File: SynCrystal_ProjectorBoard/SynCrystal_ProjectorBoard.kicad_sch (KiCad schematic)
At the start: 20 parts, among them J10 Screw_Terminal_01x03, J11 to DIN Traces, J5 Relais Board, J6 uC Cable, J7 to DIN Connector, J8 to Motor Ctrl PCB, J9 to Motor Controller Hat, SW6 SW_SPDT, U10 AP63205WU, U9 TS5A3357DCUR

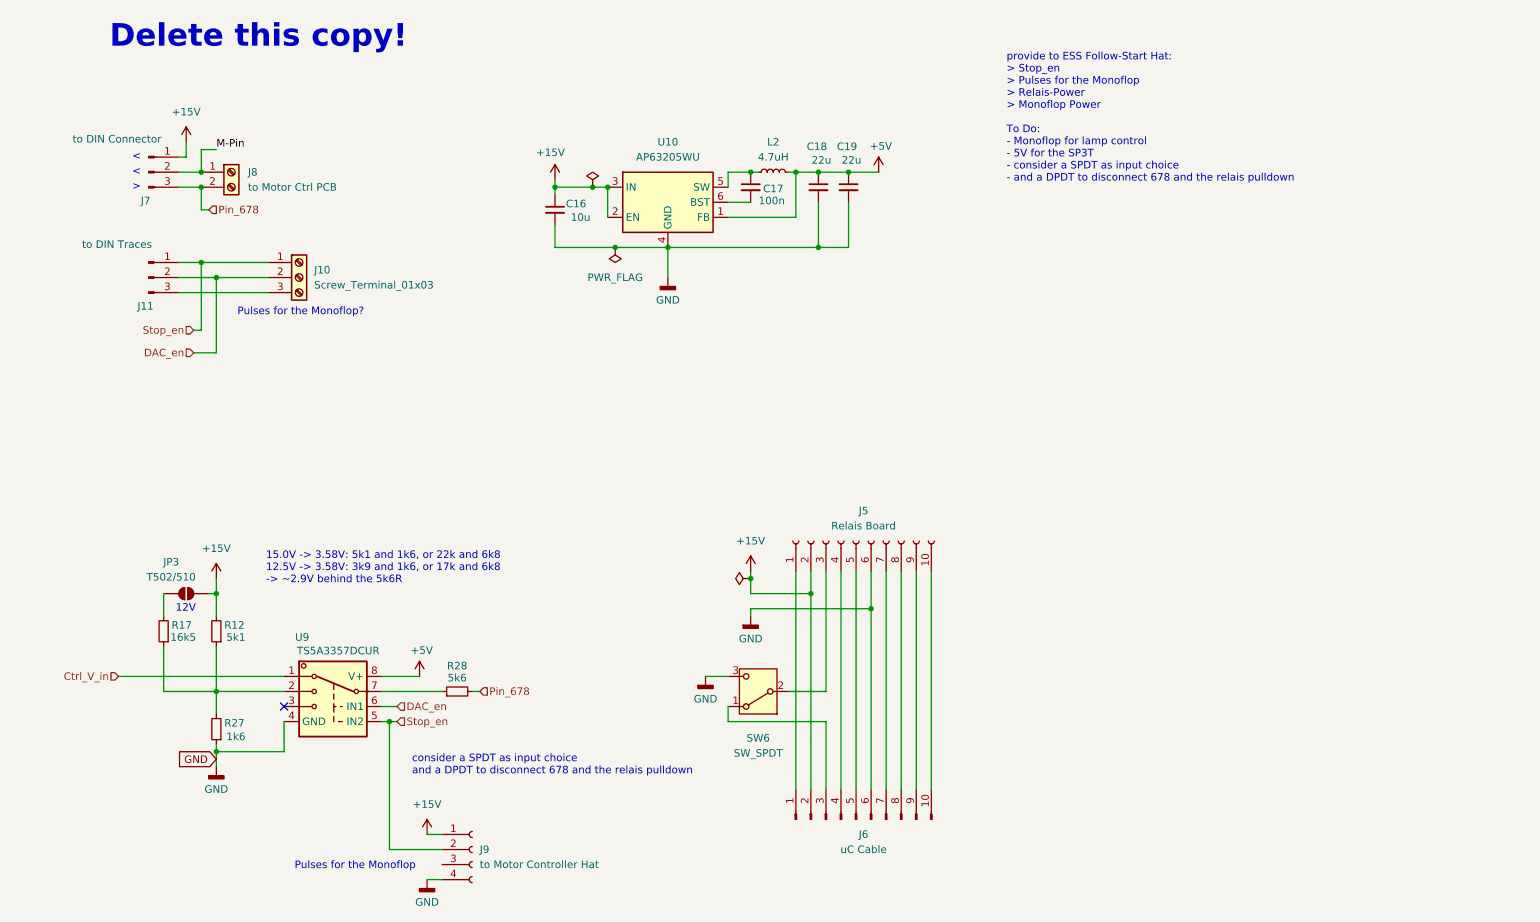
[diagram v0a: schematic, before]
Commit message: Projector PCB!
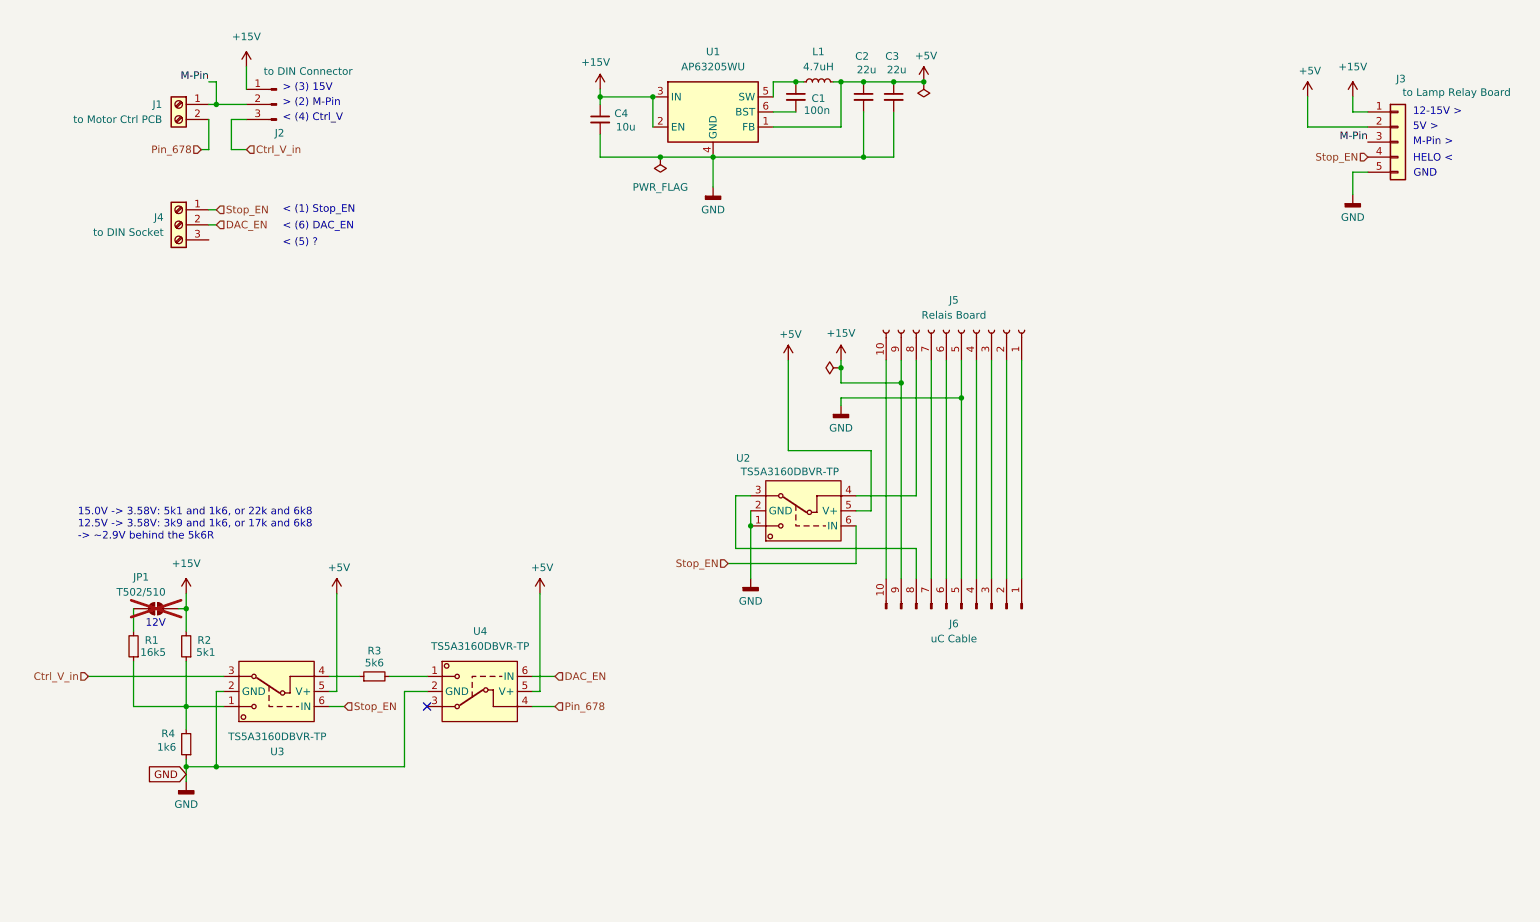
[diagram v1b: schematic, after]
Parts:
- removed J11: to DIN Traces, symbol Connector:Conn_01x03_Pin
- removed J9: to Motor Controller Hat, symbol Connector:Conn_01x04_Socket
- removed SW6: SW_SPDT, symbol Switch:SW_SPDT
- removed U9: TS5A3357DCUR, easyeda2kicad:VSSOP-8_L2.4-W2.1-P0.50-LS3.2-BR, symbol easyEDA:TS5A3357DCUR_nicer
- added J3: to Lamp Relay Board, easyEDA:CONN-TH_5P-P2.50_ZX-XH2.54-5PZZ, symbol Connector_Generic:Conn_01x05
- added U2, U3, U4: TS5A3160DBVR-TP, easyEDA:SOT-23-6_L2.9-W1.6-P0.95-LS2.8-BR, symbol easyEDA:TS5A3160DBVR-TP_nicer
- J1: renamed from J8; footprint (none) -> easyEDA:CONN-TH_2P-P2.54_MX128-2.54-GN01-02P-CU-Y-A; LCSC (none) -> C5188442
- J2: renamed from J7; footprint (none) -> Peacemans Teile:PinHeader_1x03_P2.54mm_Vertical_BAUER; LCSC (none) -> C5188443
- J4: renamed from J10; value Screw_Terminal_01x03 -> to DIN Socket; footprint (none) -> easyEDA:CONN-TH_3P-P2.54_MX128-2.54-03P-GN01-CU-Y-A; LCSC (none) -> C5188443
- J5: footprint (none) -> easyEDA:HDR-TH_10P-P2.54-H-F-W10.0-N; LCSC (none) -> C2897392
- J6: footprint (none) -> Connector_PinHeader_2.54mm:PinHeader_1x10_P2.54mm_Horizontal
- JP1: renamed from JP3; footprint (none) -> Jumper:SolderJumper-2_P1.3mm_Open_TrianglePad1.0x1.5mm; now not fitted
- renumbered C17 to C1, C18 to C2, C19 to C3, C16 to C4, L2 to L1, R17 to R1, R12 to R2, R28 to R3, R27 to R4, U10 to U1
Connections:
- net +15V: now also J5.9 (Pin_9), J6.9 (Pin_9), J3.1 (Pin_1); no longer J5.2 (Pin_2), J6.2 (Pin_2)
- net +5V: now also J3.2 (Pin_2), U2.5 (V+), U3.5 (V+), U4.5 (V+)
- net Ctrl_V_in: now also J2.3 (Pin_3), U3.3
- net GND: now also J5.5 (Pin_5), J6.5 (Pin_5), J3.5 (Pin_5), U2.1, U2.2 (GND), U3.2 (GND), U4.2 (GND); no longer J5.6 (Pin_6), J6.6 (Pin_6)
- net M-Pin: now also J3.3 (Pin_3)
- net Pin_678: now also U4.4; no longer J2.3 (Pin_3), R3.2
- net at R1.1, R2.1, R4.2: now also U3.1
- net at J5.3 (Pin_3): now also J6.3 (Pin_3)
- net at J6.8 (Pin_8): now also U2.3; no longer J5.8 (Pin_8)
- net at R3.1: now also U3.4
- net DAC_en renamed DAC_EN
- net DAC_EN: now also U4.6 (IN)
- net Stop_en renamed Stop_EN
- net Stop_EN: now also J3.4 (Pin_4), U2.6 (IN), U3.6 (IN)
- new net: J5.8 (Pin_8), U2.4
- new net: J5.2 (Pin_2), J6.2 (Pin_2)
- new net: J5.6 (Pin_6), J6.6 (Pin_6)
- new net: R3.2, U4.1
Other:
- note added: "12-15V >"
- note added: "5V >"
- note added: "< (1) Stop_EN"
- note added: "< (4) Ctrl_V"
- note added: "< (5) ?"
- note added: "< (6) DAC_EN"
- note added: "> (2) M-Pin"
- note added: "> (3) 15V"
- note added: "GND"
- note added: "HELO <"
- note added: "M-Pin >"
- note removed: "<"
- note removed: ">"
- note removed: "Delete this copy!"
- note removed: "Pulses for the Monoflop"
- note removed: "Pulses for the Monoflop?"
- note removed: "consider a SPDT as input choice and a DPDT to disconnect 678 and the relais pulldown"
- note removed: "provide to ESS Follow-Start Hat: > Stop_en > Pulses for the Monoflop > Relais-Power > Monoflop Power To Do: - Monoflop for lamp control - 5V for the SP3T - consider a SPDT as input choice - and a DPDT to disconnect 678 and the relais pulldown"
- moved on the sheet: C1, C2, C3, C4, J1, J2, J4, J5, J6, L1, R1, R2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
